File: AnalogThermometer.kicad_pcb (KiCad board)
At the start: 2 copper layers, 42.4 x 39.1 mm, 22 parts, among them P1 Power, P2 uA, P3 Vout, P4 Vtemp, Q1 MMBT3904, U1 LTC1541, U2 MCP6V11, U3 MCP9700A

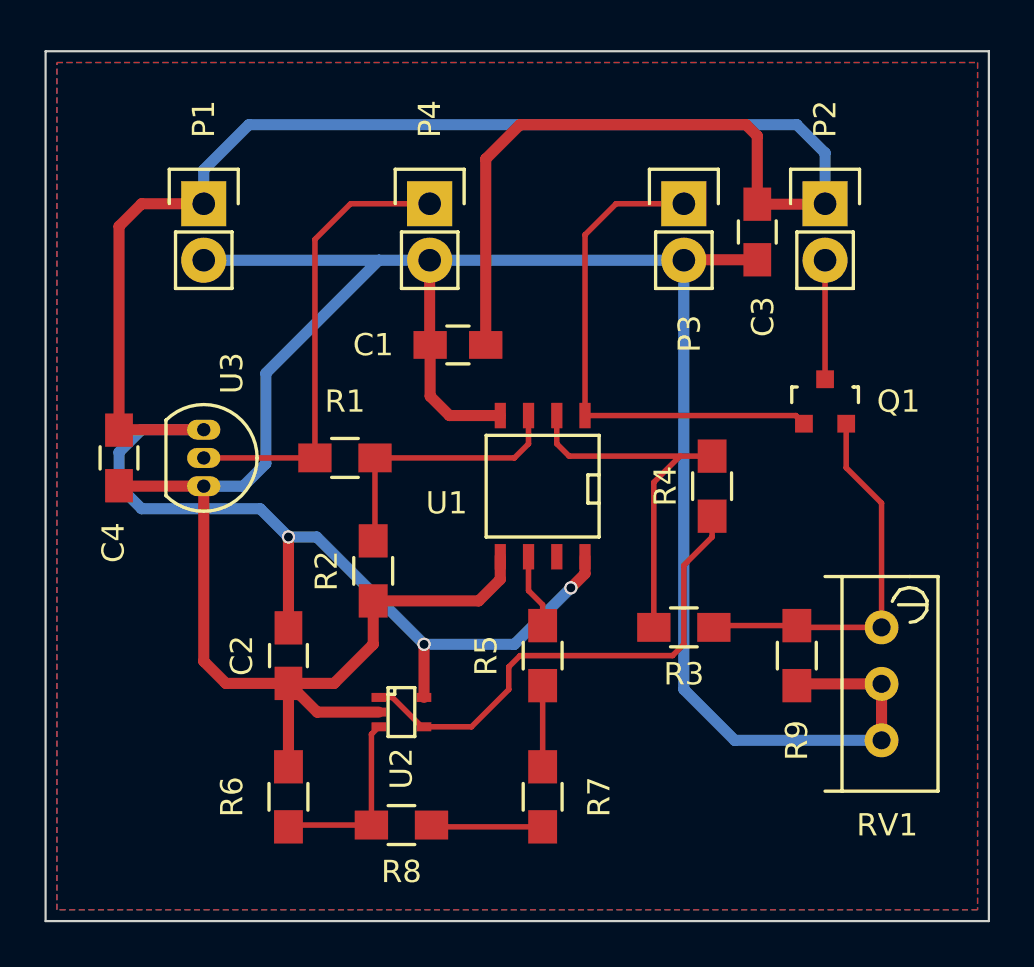
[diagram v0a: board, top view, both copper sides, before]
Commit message: Updated to rev 1.2
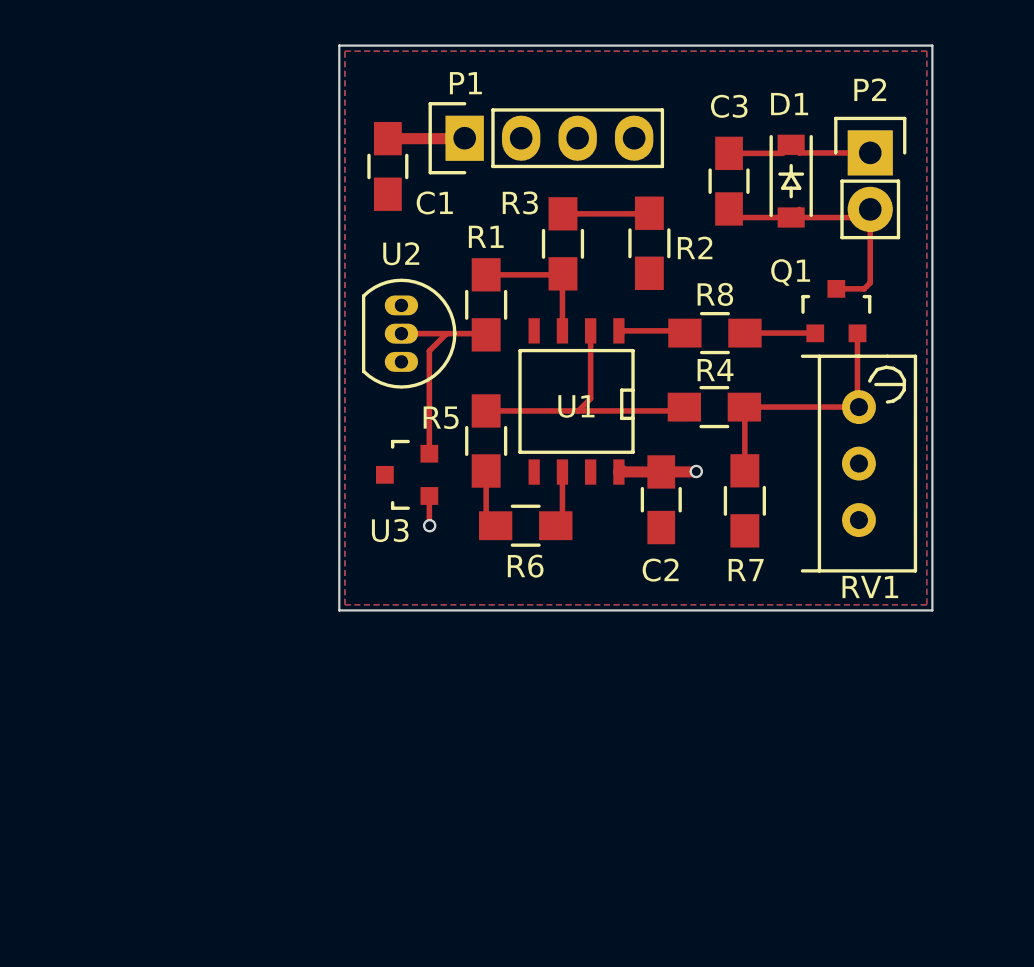
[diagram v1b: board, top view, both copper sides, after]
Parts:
- removed C4: 0.1uF, Capacitors_SMD:C_0805_HandSoldering
- removed P3: Vout, Socket_Strips:Socket_Strip_Straight_1x02
- removed P4: Vtemp, Socket_Strips:Socket_Strip_Straight_1x02
- removed R9: 33.2k, Resistors_SMD:R_0805_HandSoldering
- added D1: 1N4148, Diodes_SMD:SOD-123, F.Cu at (78.5, 98.0)
- P1: footprint Socket_Strips:Socket_Strip_Straight_1x02 -> Socket_Strips:Socket_Strip_Straight_1x04
- R2, R5: value 1M -> 2.2M
- R3, R6: value 1M -> 200k
- R7: value 200k -> 49.9k
- R8: value 200k -> 100
- U2: value MCP6V11 -> MCP9700A; footprint TO_SOT_Packages_SMD:SC-70-5 -> TO_SOT_Packages_THT:TO-92_Inline_Narrow_Oval
- U3: value MCP9700A -> MCP9700AT; footprint TO_SOT_Packages_THT:TO-92_Inline_Narrow_Oval -> TO_SOT_Packages_SMD:SOT-23
- moved R8 26.2 mm to (75.1, 104.9)
- moved U2 18.3 mm to (61.0, 103.6)
- moved C2 18.2 mm to (72.6, 112.4)
- moved R3 17.3 mm to (72.1, 100.8), turned to 90 degrees
- moved R2 17.0 mm to (68.2, 100.9), turned to 270 degrees
- moved R6 16.2 mm to (66.5, 113.5), turned to 180 degrees
- moved R7 16.1 mm to (76.4, 112.4), turned to 90 degrees
- moved P1 12.1 mm to (63.8, 96.1), turned to 0 degrees
- moved R5 9.98 mm to (64.8, 109.7)
- moved RV1 9.96 mm to (81.5, 108.2)
- moved U3 9.37 mm to (61.2, 111.3), turned to 90 degrees
- moved R1 9.37 mm to (64.8, 103.6), turned to 270 degrees
- moved C1 8.62 mm to (60.4, 97.4), turned to 90 degrees
- moved U1 4.10 mm to (68.8, 108.0)
- moved Q1 4.10 mm to (80.5, 103.9)
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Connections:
- C3 pad 1: GND -> Net-(C3-Pad1)
- P1 pad 2: GND -> Net-(P1-Pad2)
- P2 pad 2: Net-(P2-Pad2) -> Net-(C3-Pad1)
- Q1 pad 1: Net-(P3-Pad1) -> Net-(Q1-Pad1)
- Q1 pad 3: Net-(P2-Pad2) -> Net-(C3-Pad1)
- R1 pad 2: Net-(P4-Pad1) -> Net-(R1-Pad2)
- R2 pad 1: GND -> Net-(R2-Pad1)
- R3 pad 1: Net-(Q1-Pad2) -> GND
- R3 pad 2: Net-(R3-Pad2) -> Net-(R2-Pad1)
- R4 pad 1: Net-(R4-Pad1) -> Net-(Q1-Pad2)
- R4 pad 2: Net-(R3-Pad2) -> Net-(R4-Pad2)
- R5 pad 2: Net-(R5-Pad2) -> Net-(R4-Pad2)
- R6 pad 1: GND -> Net-(R6-Pad1)
- R6 pad 2: Net-(R6-Pad2) -> Net-(R5-Pad1)
- R7 pad 1: Net-(R5-Pad1) -> GND
- R7 pad 2: Net-(R7-Pad2) -> Net-(Q1-Pad2)
- R8 pad 1: Net-(R7-Pad2) -> Net-(Q1-Pad1)
- R8 pad 2: Net-(R6-Pad2) -> Net-(R8-Pad2)
- U1 pad 1: Net-(P3-Pad1) -> Net-(R8-Pad2)
- U1 pad 2: Net-(R3-Pad2) -> Net-(R4-Pad2)
- U1 pad 6: Net-(R5-Pad2) -> Net-(R6-Pad1)
- U2 pad 1: Net-(R4-Pad1) -> +5V
- U2 pad 2: GND -> Net-(R1-Pad2)
- U2 pad 3: Net-(R6-Pad2) -> GND
- U3 pad 2: Net-(P4-Pad1) -> Net-(R1-Pad2)
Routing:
- net GND: track 122.5 -> 0.00 mm
- net +5V: track 116.1 -> 15.1 mm, vias 3 -> 2
- net Net-(P3-Pad1): track 23.1 -> 0.00 mm
- net Net-(R4-Pad1): track 22.7 -> 0.00 mm
- net Net-(P4-Pad1): track 20.7 -> 0.00 mm
- net Net-(R3-Pad2): track 16.7 -> 0.00 mm
- net Net-(R4-Pad2): track 0.00 -> 13.1 mm
- net Net-(C3-Pad1): track 0.00 -> 12.1 mm
- net Net-(R1-Pad2): track 0.00 -> 9.62 mm
- net Net-(R6-Pad2): track 8.43 -> 0.00 mm
- net Net-(Q1-Pad2): track 17.7 -> 11.4 mm
- net Net-(R1-Pad1): track 12.2 -> 5.94 mm
- net Net-(P2-Pad2): track 5.35 -> 0.00 mm
- net Net-(R7-Pad2): track 5.15 -> 0.00 mm
- net Net-(R2-Pad1): track 0.00 -> 3.90 mm
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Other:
- board size 42.4 x 39.1 mm -> 26.7 x 25.4 mm
- board text added: "http://www.analogzoo.com"
